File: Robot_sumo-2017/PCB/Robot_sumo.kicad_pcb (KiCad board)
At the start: 2 copper layers, 58 parts, among them J1 CONN_Batt, J2 CONN_C1, J3 CONN_C3, J4 CONN_C2, J5 CONN_C4, J6 CONN_M1, J7 CONN_M2, J8 CONN_distance, U1 Arduino-nano, U2 LM324, U3 NE555, U4 L293

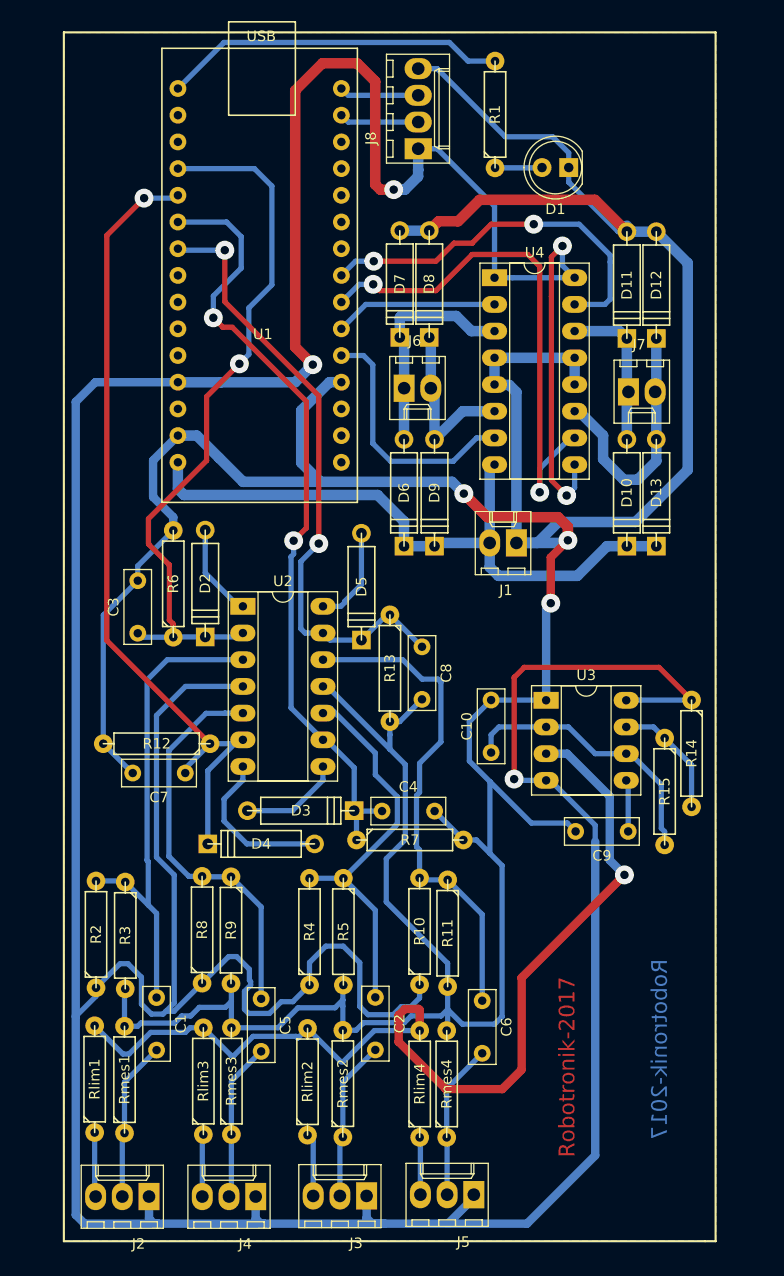
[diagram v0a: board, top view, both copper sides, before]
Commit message: last version I hope
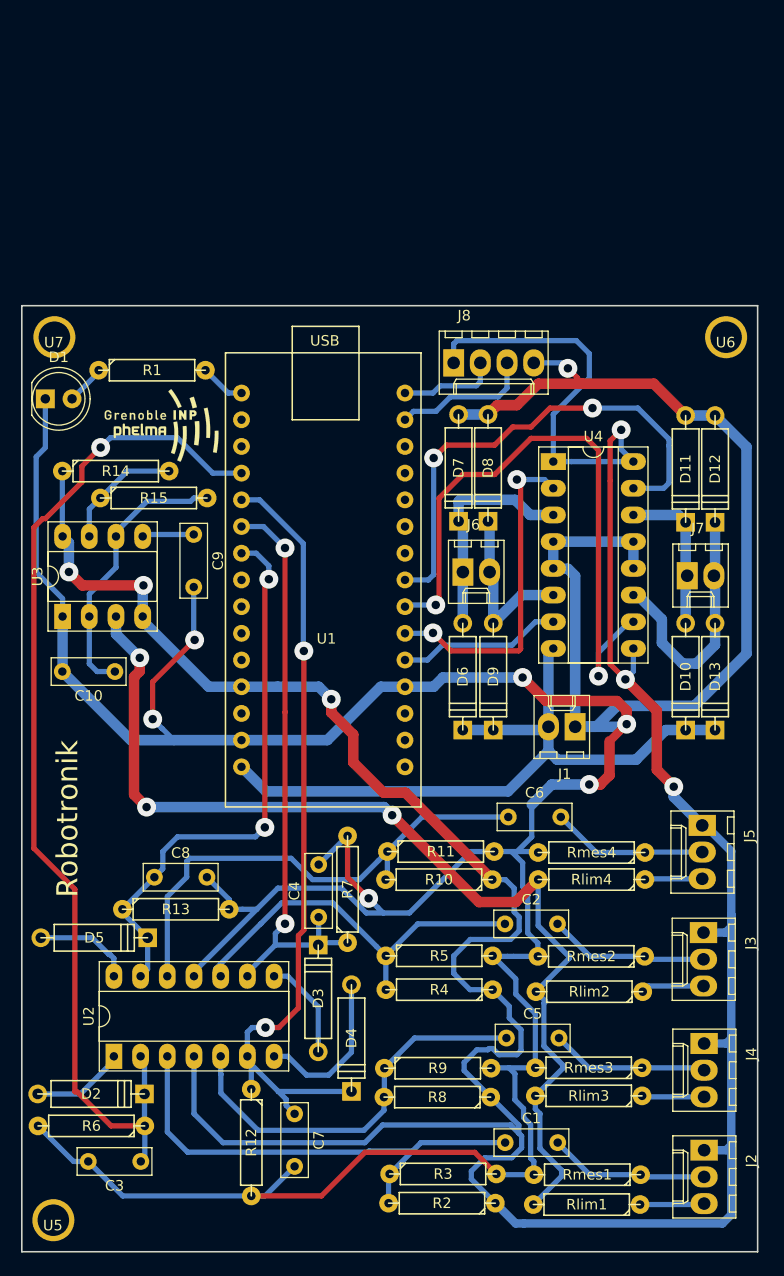
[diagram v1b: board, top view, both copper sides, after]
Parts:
- added G***: LOGO, logo:phelma-logo-exp2, B.Cu at (141.3, 126.1)
- added G***: LOGO, logo:phelma-logo, F.Cu at (118.3, 101.4)
- added U5: trou-3, Arduino-nano:Trou-3, F.Cu at (107.9, 177.0)
- added U6: trou-3, Arduino-nano:Trou-3, F.Cu at (171.9, 93.0)
- added U7: trou-3, Arduino-nano:Trou-3, F.Cu at (108.0, 93.0)
- moved R14 61.0 mm to (113.9, 105.7), turned to 0 degrees
- moved R15 56.0 mm to (117.6, 108.3), turned to 0 degrees
- moved D1 54.4 mm to (107.2, 98.9), turned to 0 degrees
- moved J2 53.0 mm to (169.9, 170.3), turned to 270 degrees
- moved R6 52.2 mm to (111.6, 168.0), turned to 180 degrees
- moved C3 50.3 mm to (116.3, 171.4), turned to 180 degrees
- moved C9 50.1 mm to (121.4, 111.8), turned to 270 degrees
- moved D2 49.8 mm to (111.6, 165.0), turned to 0 degrees
- moved Rlim1 48.3 mm to (158.7, 175.5), turned to 180 degrees
- moved U3 46.7 mm to (108.9, 119.6), turned to 90 degrees
- moved J4 45.1 mm to (169.9, 160.2), turned to 270 degrees
- moved Rmes1 44.9 mm to (158.8, 172.7), turned to 180 degrees
- moved U2 44.5 mm to (113.8, 161.4), turned to 90 degrees
- moved D5 42.0 mm to (111.9, 150.1), turned to 0 degrees
- moved R2 41.7 mm to (145.0, 175.4), turned to 180 degrees
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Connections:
- U1 pad 29: /distance_sensor/Trig -> /distance_sensor/Echo
- U1 pad 30: /distance_sensor/Echo -> /distance_sensor/Trig
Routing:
- net +5V: track 448.9 -> 315.0 mm, vias 5 -> 6
- net /R-IR/C1: track 68.7 -> 99.2 mm
- net Net-(R1-Pad2): track 32.7 -> 4.33 mm
- net /R-IR/C3: track 74.3 -> 56.5 mm
- net /motor-part/PWM1: track 15.5 -> 31.9 mm, vias 0 -> 2
- net /motor-part/PWM2: track 36.6 -> 47.4 mm
- net /motor-part/O2: track 50.0 -> 59.5 mm
- net /motor-part/O1: track 24.0 -> 15.6 mm
- net /distance_sensor/Echo: track 7.58 -> 13.4 mm
- net /R-IR/C4: track 59.2 -> 53.5 mm
- net VCC: track 63.6 -> 67.3 mm
- net /R-IR/Signal-e: track 97.8 -> 100.0 mm, vias 1 -> 3
- net /distance_sensor/Trig: track 7.58 -> 9.41 mm
- net /R-IR/C2: track 79.3 -> 77.7 mm, vias 1 -> 2
- net Net-(C6-Pad1): track 47.4 -> 48.5 mm
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- removed copper zone on B.Cu, net GND
- removed copper zone on F.Cu, net GND
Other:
- board outline added: 70 x 90 mm
- net class Default: clearance 0.254 -> 0.31
- rule trace_clearance: 0.254 -> 0.31
- board text added: "Robotronik"
- board text removed: "Robotronik-2017"
